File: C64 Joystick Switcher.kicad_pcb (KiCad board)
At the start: 2 copper layers, 49.3 x 81.9 mm, 30 parts, among them J1 Port 1, J2 Port 2, J3 Joystick, J4 B2_SEL, J5 B1_SEL, Q1 BC547, SW1 P1_SEL, SW2 P2_SEL, U1 74HCT4053, U2 74HCT4053, U3 NE555, U4 NE555

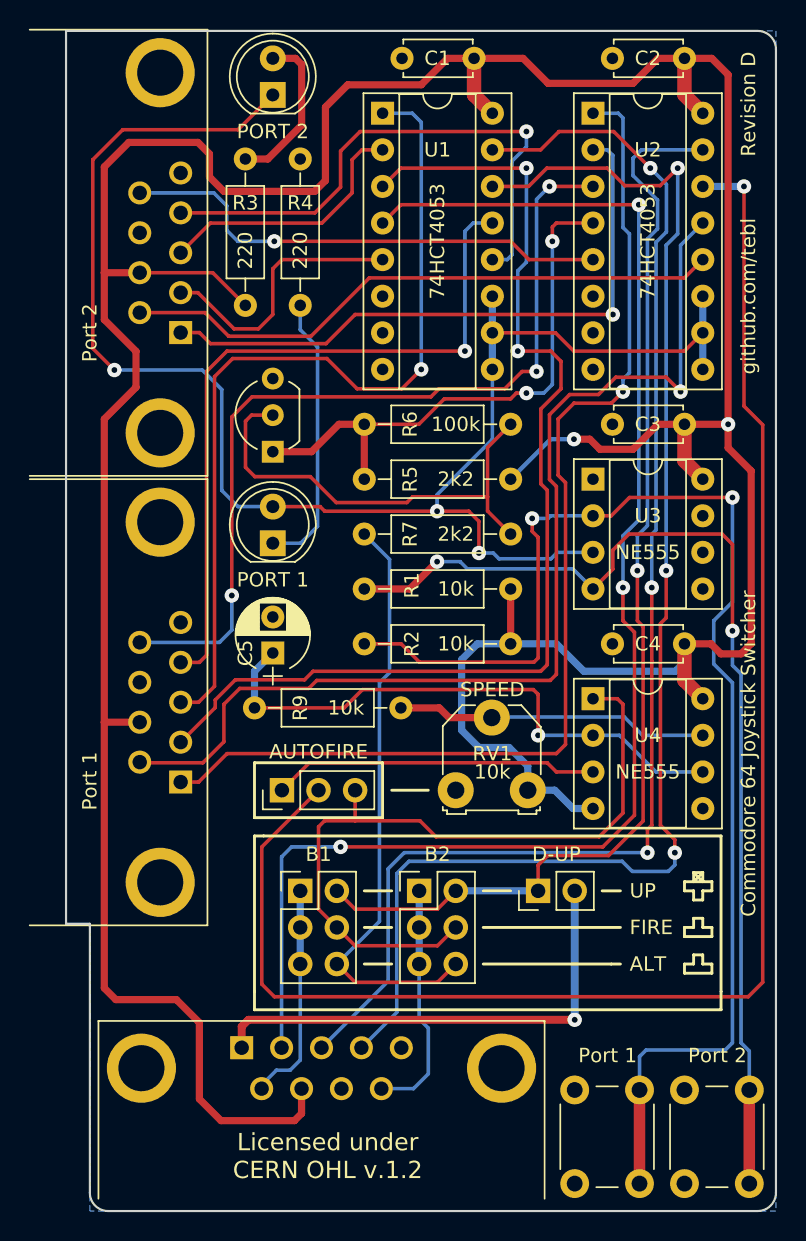
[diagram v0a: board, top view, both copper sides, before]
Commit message: Layout done. PCB ready for manufacturing.
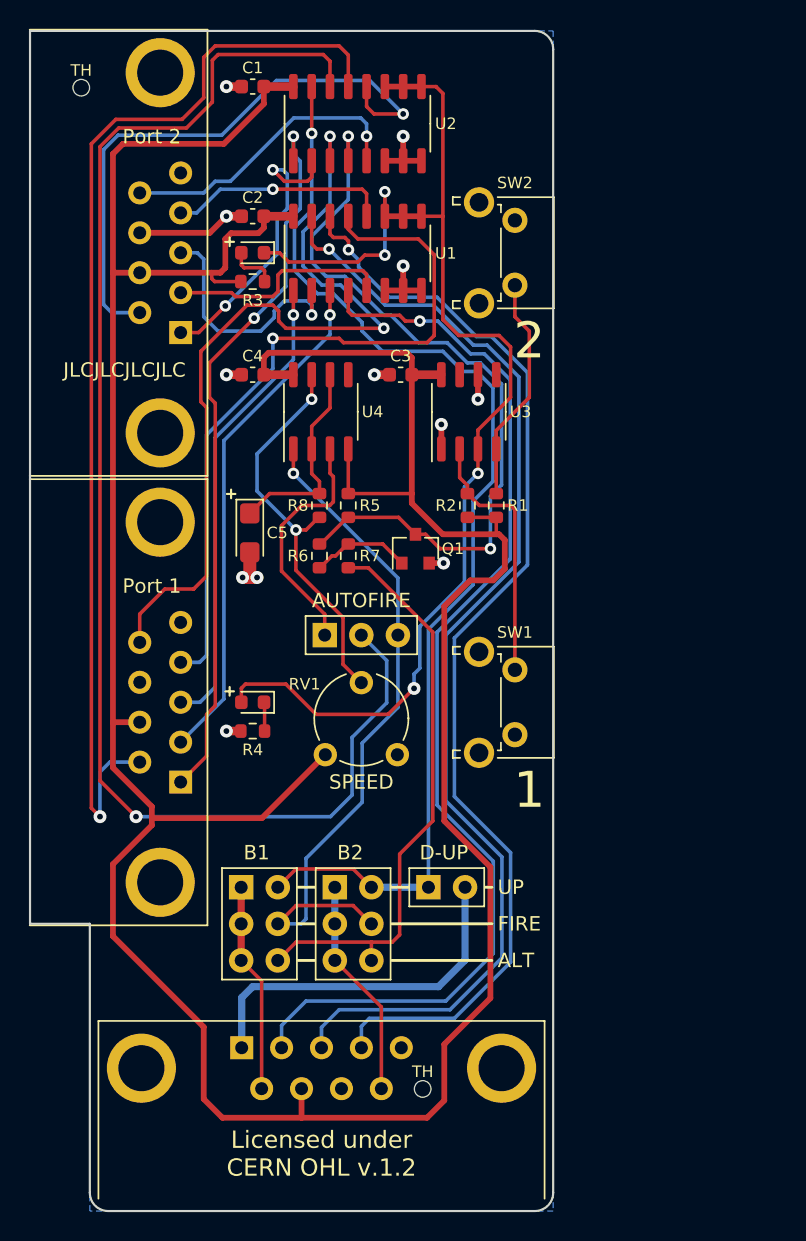
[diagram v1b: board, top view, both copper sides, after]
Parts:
- added TH: Tooling Hole 1,1mm, MountingHole:MountingHole_2.1mm, F.Cu at (122.8, 109.0)
- added TH: Tooling Hole 1,1mm, MountingHole:MountingHole_2.1mm, F.Cu at (99.1, 39.5)
- C1, C2, C3, C4: footprint Capacitors_THT:C_Disc_D4.7mm_W2.5mm_P5.00mm -> Capacitor_SMD:C_0603_1608Metric
- C5: footprint Capacitors_THT:CP_Radial_D5.0mm_P2.50mm -> Capacitor_Tantalum_SMD:CP_EIA-3216-18_Kemet-A
- D1, D2: footprint LEDs:LED_D5.0mm -> LED_SMD:LED_0603_1608Metric
- Q1: value BC547 -> BC847; footprint TO_SOT_Packages_THT:TO-92_Inline_Wide -> Package_TO_SOT_SMD:SOT-23
- R1, R2, R3, R4, R5, R6, R7: footprint Resistors_THT:R_Axial_DIN0207_L6.3mm_D2.5mm_P10.16mm_Horizontal -> Resistor_SMD:R_0603_1608Metric
- R8: renamed from R9; footprint Resistors_THT:R_Axial_DIN0207_L6.3mm_D2.5mm_P10.16mm_Horizontal -> Resistor_SMD:R_0603_1608Metric
- RV1: footprint Potentiometers:Potentiometer_Triwood_RM-065 -> Potentiometer_THT:Potentiometer_Piher_PT-6-V_Vertical
- SW1, SW2: footprint Buttons_Switches_THT:SW_PUSH_6mm -> Button_Switch_THT:SW_Tactile_SPST_Angled_PTS645Vx58-2LFS
- U1, U2: value 74HCT4053 -> 74HCT4053D; footprint Housings_DIP:DIP-16_W7.62mm_Socket -> Package_SO:SO-16_3.9x9.9mm_P1.27mm
- U3, U4: value NE555 -> TLC555CDR; footprint Housings_DIP:DIP-8_W7.62mm_Socket -> Package_SO:SO-8_3.9x4.9mm_P1.27mm
- moved SW2 67.9 mm to (129.2, 48.7), turned to 270 degrees
- moved R4 39.8 mm to (111.0, 84.2), turned to 0 degrees
- moved SW1 35.9 mm to (129.2, 79.9), turned to 270 degrees
- moved C4 35.3 mm to (111.0, 59.4)
- moved C2 31.9 mm to (111.0, 48.4)
- moved U4 27.4 mm to (115.7, 62.0), turned to 90 degrees
- moved C3 20.0 mm to (121.3, 59.4)
- moved U2 16.4 mm to (118.3, 42.0), turned to 90 degrees
- moved C1 15.5 mm to (111.0, 39.4)
- moved R8 14.8 mm to (115.6, 68.5), turned to 270 degrees
- moved R2 12.0 mm to (125.9, 68.5), turned to 270 degrees
- moved Q1 12.0 mm to (122.3, 71.5)
- moved JP2 11.2 mm to (116.0, 77.5)
- moved D2 11.1 mm to (111.0, 82.2), turned to 180 degrees
- moved D1 11.0 mm to (111.0, 51.0), turned to 180 degrees
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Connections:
- J1 pad 5: (no net) -> Net-(J1-Pad5)
- J2 pad 5: (no net) -> Net-(J2-Pad5)
- J3 pad 5: (no net) -> Net-(J3-Pad5)
- Q1 pad 1: ALT_FIRE -> Net-(Q1-Pad1)
- Q1 pad 2: Net-(Q1-Pad2) -> GND
- Q1 pad 3: GND -> ALT_FIRE
- R6 pad 2: Net-(Q1-Pad2) -> Net-(Q1-Pad1)
- R7 pad 2: Net-(Q1-Pad2) -> Net-(Q1-Pad1)
- RV1 pad 1: (no net) -> Net-(RV1-Pad1)
- SW1 pad 1: GND -> Net-(R2-Pad1)
- SW1 pad 2: Net-(R2-Pad1) -> GND
- U3 pad 5: (no net) -> Net-(U3-Pad5)
- U3 pad 7: (no net) -> Net-(U3-Pad7)
- U4 pad 5: (no net) -> Net-(U4-Pad5)
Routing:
- net Net-(R2-Pad1): track 91.7 -> 18.2 mm, vias 2 -> 0
- net Net-(R1-Pad1): track 74.6 -> 15.8 mm, vias 2 -> 0
- net VCC: track 269.5 -> 227.8 mm, vias 2 -> 0
- net Net-(J1-Pad2): track 76.6 -> 35.6 mm, vias 2 -> 1
- net Net-(Q1-Pad2): track 32.2 -> 0.00 mm
- net Net-(J1-Pad3): track 60.7 -> 32.6 mm
- net GND: track 0.00 -> 27.3 mm, vias 0 -> 12
- net Net-(J1-Pad1): track 77.5 -> 50.5 mm, vias 1 -> 2
- net Net-(C5-Pad1): track 40.6 -> 14.4 mm, vias 1 -> 0
- net PORT: track 111.0 -> 85.6 mm, vias 3 -> 4
- net DOWN: track 100.4 -> 76.5 mm, vias 3 -> 1
- net Net-(J2-Pad4): track 38.9 -> 15.3 mm
- net Net-(J2-Pad1): track 43.7 -> 20.2 mm, vias 1 -> 2
- net RIGHT: track 97.4 -> 78.4 mm, vias 3 -> 1
- net Net-(D2-Pad1): track 19.4 -> 2.02 mm
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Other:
- board size 49.3 x 81.9 mm -> 36.3 x 81.9 mm
- board text added: "1"
- board text added: "2"
- board text added: "Do NOT change when powered, do not jumper more than one per line!"
- board text added: "Enable AF"
- board text added: "JLCJLCJLCJLC"
- board text added: "Original circuit by: github.com/tebl SMD-PCB by: github.com/ttahsin-bey"
- board text added: "SMD-Rev. A"
- board text removed: "10k"
- board text removed: "Do NOT change when powered, do not jumper more than once per line!"
- board text removed: "ENABLE"
- board text removed: "PORT 1"
- board text removed: "PORT 2"
- board text removed: "Port 1"
- board text removed: "Port 2"
- board text removed: "Revision D"
- board text removed: "github.com/tebl"
